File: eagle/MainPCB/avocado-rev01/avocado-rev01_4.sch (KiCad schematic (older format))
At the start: 2 parts, among them U1 V3S

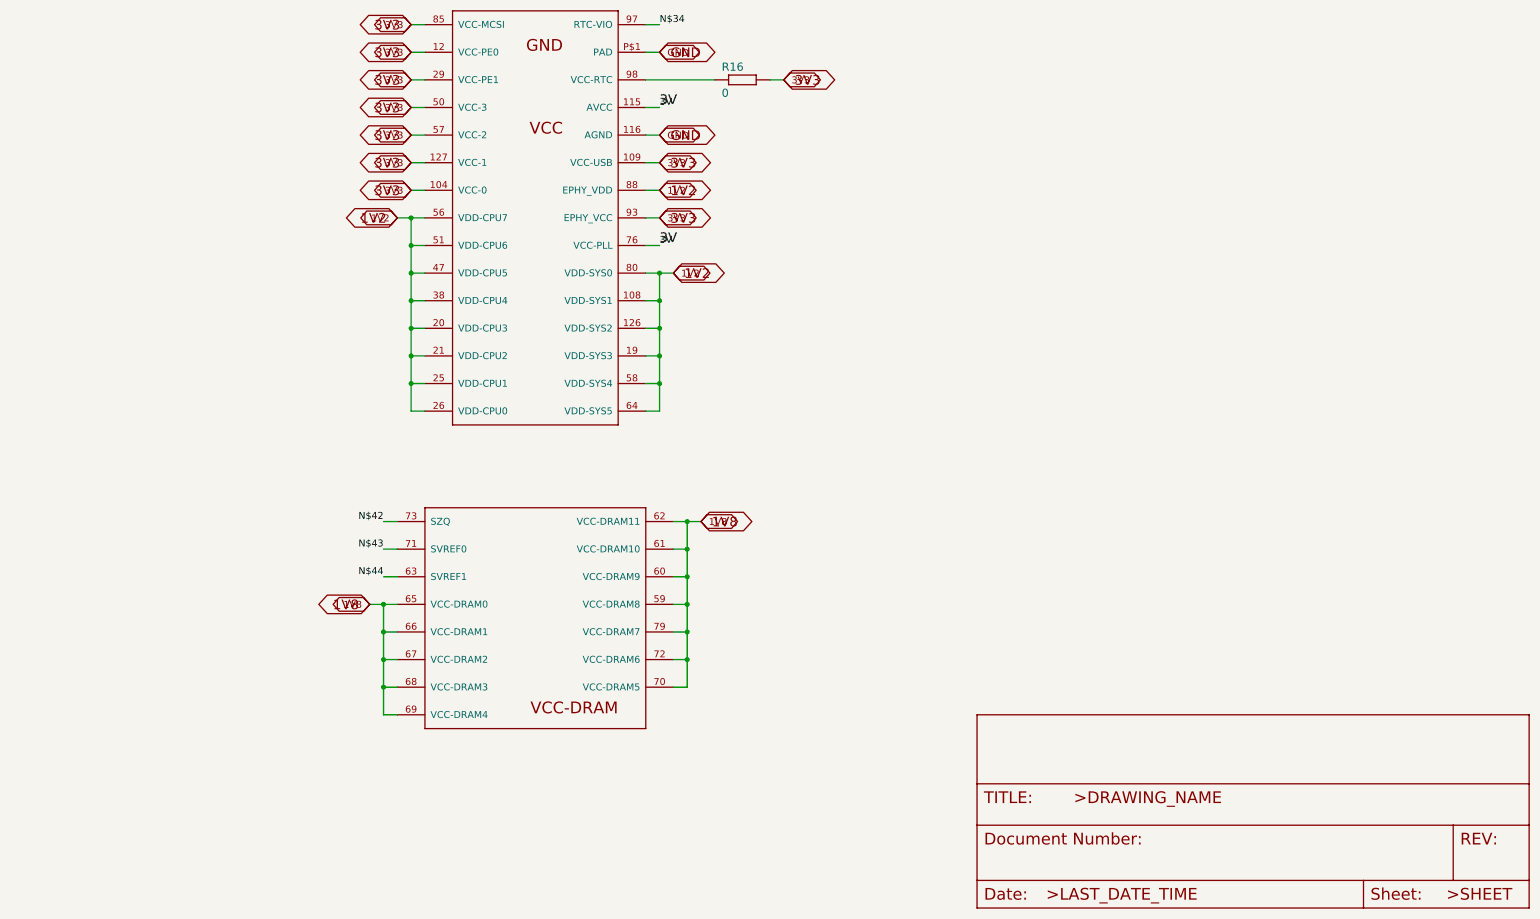
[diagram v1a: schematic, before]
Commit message: decoupling caps
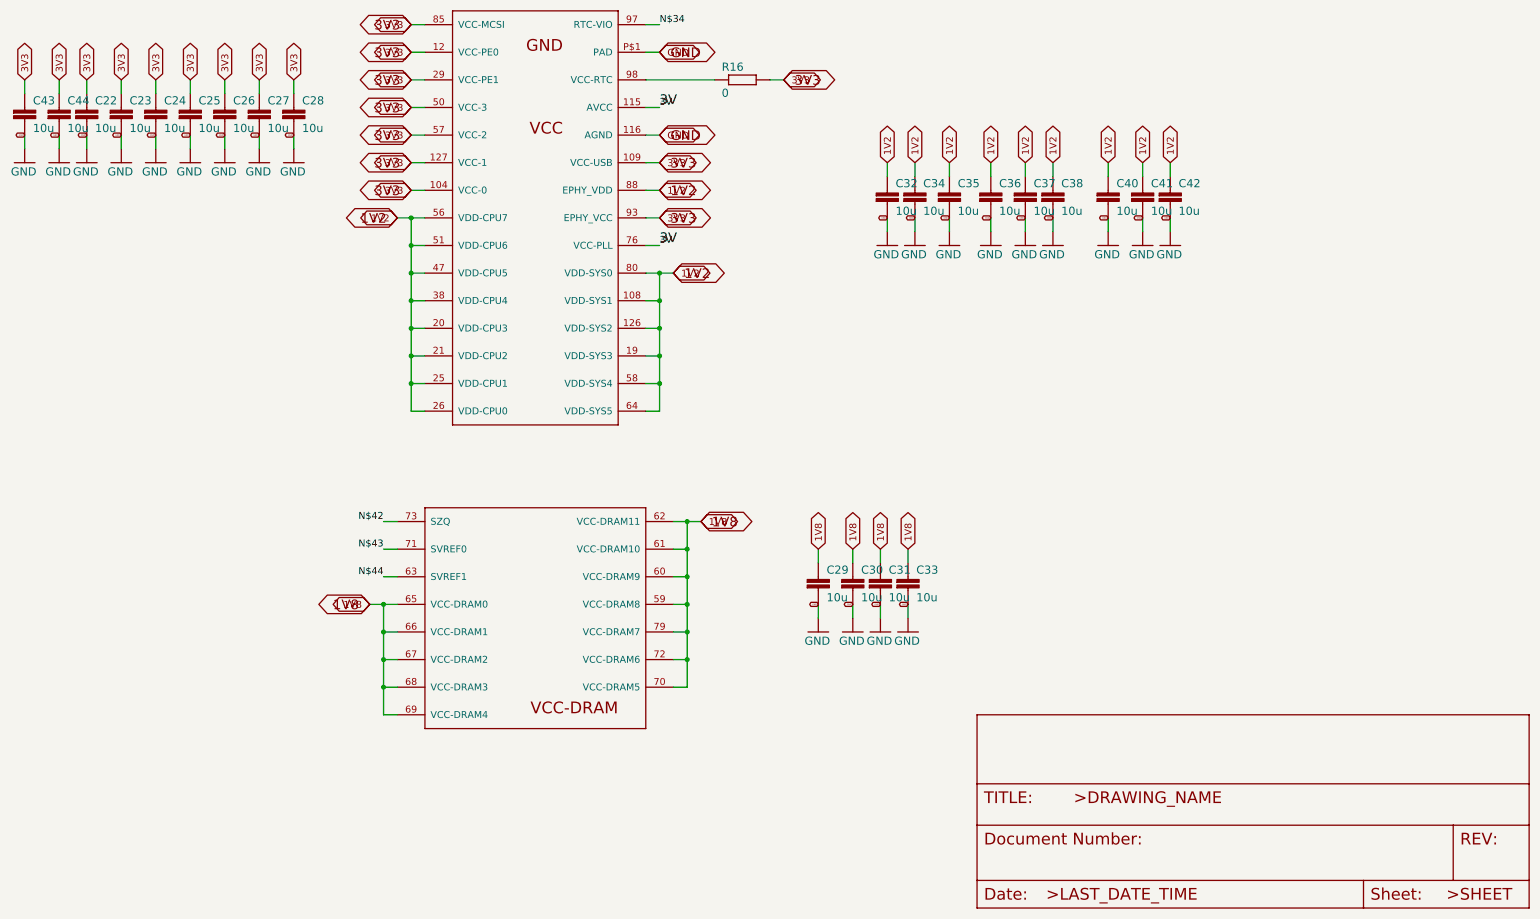
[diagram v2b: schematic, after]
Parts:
- added C22, C23, C24, C25, C26, C27, C28, C29, C30, C31, C32, C33, C34, C35, C36, C37, C38, C40, C41, C42, C43, C44: 10u, avocado-rev01:C0603, symbol avocado-rev01-eagle-import:C0603
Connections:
- net 1V2: now also C32.1, C34.1, C35.1, C36.1, C37.1, C38.1, C40.1, C41.1, C42.1
- net 1V8: now also C29.1, C30.1, C31.1, C33.1
- net 3V3: now also C22.1, C23.1, C24.1, C25.1, C26.1, C27.1, C28.1, C43.1, C44.1
- net GND: now also C22.2, C23.2, C24.2, C25.2, C26.2, C27.2, C28.2, C29.2, C30.2, C31.2, C32.2, C33.2, C34.2, C35.2, C36.2, C37.2, C38.2, C40.2, C41.2, C42.2, C43.2, C44.2
